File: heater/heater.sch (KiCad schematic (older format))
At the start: 9 parts, among them J1 power Input, J2 input uC, J3 thermostat, J4 to mcu, Q1 BC517

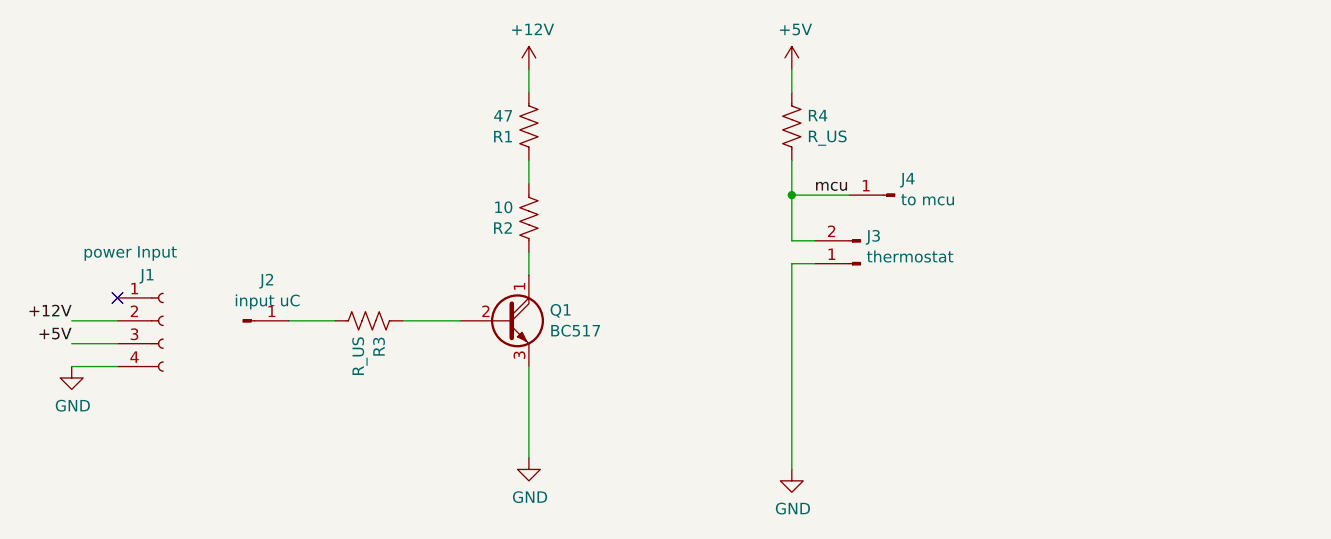
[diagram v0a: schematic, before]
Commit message: heater done
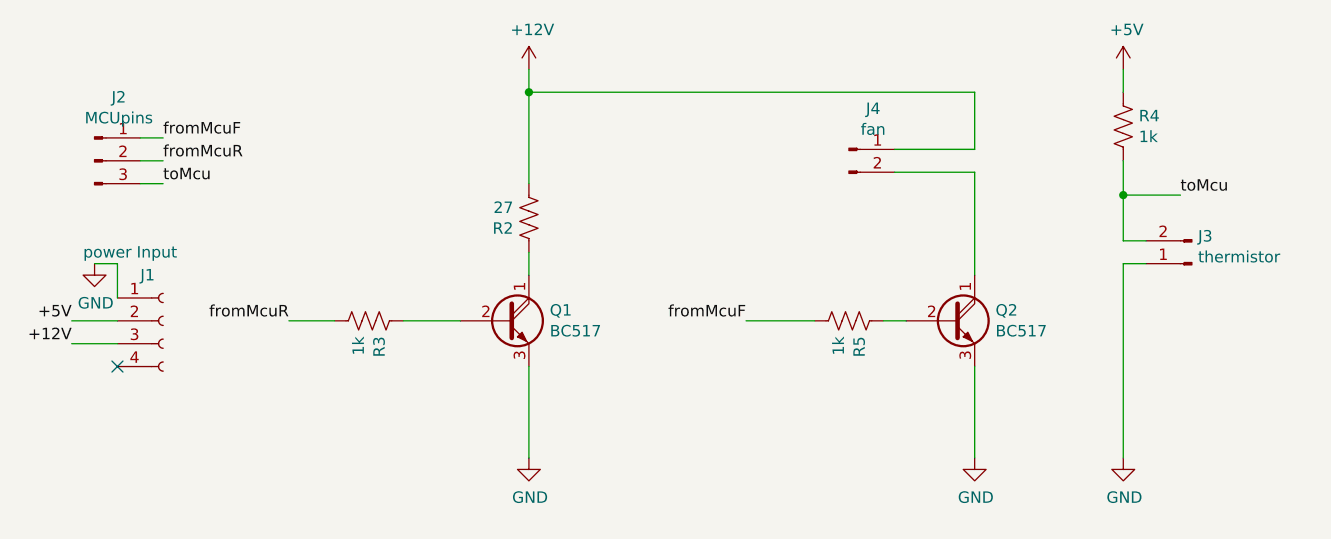
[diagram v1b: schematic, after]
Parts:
- removed J2: input uC, Socket_Strips:Socket_Strip_Straight_1x01_Pitch2.54mm, symbol Connector:Conn_01x01_Male
- removed J4: to mcu, Socket_Strips:Socket_Strip_Straight_1x01_Pitch2.54mm, symbol Connector:Conn_01x01_Male
- removed R1: 47, Resistors_THT:R_Axial_DIN0414_L11.9mm_D4.5mm_P15.24mm_Horizontal, symbol Device:R_US
- added J2: MCUpins, Connectors_JST:JST_XH_B03B-XH-A_03x2.50mm_Straight, symbol Connector:Conn_01x03_Male
- added J4: fan, Connectors_JST:JST_XH_B02B-XH-A_02x2.50mm_Straight, symbol Connector:Conn_01x02_Male
- added Q2: BC517, TO_SOT_Packages_THT:TO-92_Inline_Wide, symbol Transistor_BJT:BC517
- added R5: 1k, Resistors_SMD:R_0805_HandSoldering, symbol Device:R_US
- J1: footprint Connectors_JST:JST_EH_B04B-EH-A_04x2.50mm_Straight -> Connectors_JST:JST_XH_B04B-XH-A_04x2.50mm_Straight
- J3: value thermostat -> thermistor; footprint Socket_Strips:Socket_Strip_Straight_1x02_Pitch2.54mm -> Connectors_JST:JST_XH_B02B-XH-A_02x2.50mm_Straight
- R2: value 10 -> 27; footprint Resistors_THT:R_Axial_Power_L75.0mm_W9.0mm_P81.28mm -> Resistors_THT:R_Axial_Power_L38.0mm_W9.0mm_P40.64mm
- R3, R4: value R_US -> 1k
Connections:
- net +12V: now also J1.3 (Pin_3), R2.2, J4.1 (Pin_1); no longer J1.2 (Pin_2)
- net +5V: now also J1.2 (Pin_2); no longer J1.3 (Pin_3)
- net GND: now also J1.1 (Pin_1), Q2.3 (E); no longer J1.4 (Pin_4)
- net fromMcuR: now reaches R3.2
- net fromMcuR: now also J2.2 (Pin_2)
- net mcu renamed toMcu
- net toMcu: now also J2.3 (Pin_3)
- new net: J4.2 (Pin_2), Q2.1 (C)
- new net: Q2.2 (B), R5.1
- new net fromMcuF: J2.1 (Pin_1), R5.2
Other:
- moved on the sheet: J3, R4
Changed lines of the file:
@@
 P 3750 2050
 F 0 "R2" H 3818 2096 50  0000 L CNN
-F 1 "10" H 3818 2005 50  0000 L CNN
-F 2 "Resistors_THT:R_Axial_Power_L75.0mm_W9.0mm_P81.28mm" V 3790 2040 50  0001 C CNN
+F 1 "27" H 3818 2005 50  0000 L CNN
+F 2 "Resistors_THT:R_Axial_Power_L38.0mm_W9.0mm_P40.64mm" V 3790 2040 50  0001 C CNN
 F 3 "~" H 3750 2050 50  0001 C CNN
 	1    3750 2050
-	-1   0    0    1
-$EndComp
-$Comp
-L Device:R_US R1
-U 1 1 5C2F3120
-P 3750 1650
-F 0 "R1" H 3818 1696 50  0000 L CNN
-F 1 "47" H 3818 1605 50  0000 L CNN
-F 2 "Resistors_THT:R_Axial_DIN0414_L11.9mm_D4.5mm_P15.24mm_Horizontal" V 3790 1640 50  0001 C CNN
-F 3 "~" H 3750 1650 50  0001 C CNN
-	1    3750 1650
 	-1   0    0    1
 $EndComp
@@
 F 0 "J1" H 2050 2700 50  0000 L CNN
 F 1 "power Input" H 1800 2800 50  0000 L CNN
-F 2 "Connectors_JST:JST_EH_B04B-EH-A_04x2.50mm_Straight" H 2150 2500 50  0001 C CNN
+F 2 "Connectors_JST:JST_XH_B04B-XH-A_04x2.50mm_Straight" H 2150 2500 50  0001 C CNN
 F 3 "~" H 2150 2500 50  0001 C CNN
 	1    2150 2500
 	1    0    0    -1
 $EndComp
-Wire Wire Line
-	1950 2500 1750 2500
-Wire Wire Line
-	1950 2600 1750 2600
-Wire Wire Line
-	1950 2700 1750 2700
 Text Label 1750 2500 2    50   ~ 0
-+12V
-Text Label 1750 2600 2    50   ~ 0
 +5V
 $Comp
 L power:GND #PWR0101
 U 1 1 5C303485
-P 1750 2700
-F 0 "#PWR0101" H 1750 2450 50  0001 C CNN
-F 1 "GND" H 1755 2527 50  0000 C CNN
-F 2 "" H 1750 2700 50  0001 C CNN
-F 3 "" H 1750 2700 50  0001 C CNN
-	1    1750 2700
-	1    0    0    -1
-$EndComp
-NoConn ~ 1950 2400
+P 1850 2250
+F 0 "#PWR0101" H 1850 2000 50  0001 C CNN
+F 1 "GND" H 1855 2077 50  0000 C CNN
+F 2 "" H 1850 2250 50  0001 C CNN
+F 3 "" H 1850 2250 50  0001 C CNN
+	1    1850 2250
+	1    0    0    -1
+$EndComp
 $Comp
 L Transistor_BJT:BC517 Q1
@@
 $EndComp
 $Comp
-L Connector:Conn_01x01_Male J2
-U 1 1 5C307D7B
-P 2500 2500
-F 0 "J2" H 2606 2678 50  0000 C CNN
-F 1 "input uC" H 2606 2587 50  0000 C CNN
-F 2 "Socket_Strips:Socket_Strip_Straight_1x01_Pitch2.54mm" H 2500 2500 50  0001 C CNN
-F 3 "~" H 2500 2500 50  0001 C CNN
-	1    2500 2500
-	1    0    0    -1
-$EndComp
-$Comp
 L Device:R_US R3
 U 1 1 5C307DD4
 P 3050 2500
 F 0 "R3" H 3118 2546 50  0000 L CNN
-F 1 "R_US" H 3118 2455 50  0000 L CNN
+F 1 "1k" H 3118 2455 50  0000 L CNN
 F 2 "Resistors_SMD:R_0805_HandSoldering" V 3090 2490 50  0001 C CNN
 F 3 "~" H 3050 2500 50  0001 C CNN
@@
 	3200 2500 3450 2500
 Wire Wire Line
-	3750 1800 3750 1900
-Wire Wire Line
-	3750 2200 3750 2300
-Wire Wire Line
-	3750 1500 3750 1400
+	3750 2700 3750 3100
+$Comp
+L power:GND #PWR0103
+U 1 1 5C308243
+P 3750 3100
+F 0 "#PWR0103" H 3750 2850 50  0001 C CNN
+F 1 "GND" H 3755 2927 50  0000 C CNN
+F 2 "" H 3750 3100 50  0001 C CNN
+F 3 "" H 3750 3100 50  0001 C CNN
+	1    3750 3100
+	1    0    0    -1
+$EndComp
+$Comp
+L Connector:Conn_01x02_Male J3
+U 1 1 5C308B5A
+P 6650 2250
+F 0 "J3" H 6623 2130 50  0000 R CNN
+F 1 "thermistor" H 6623 2221 50  0000 R CNN
+F 2 "Connectors_JST:JST_XH_B02B-XH-A_02x2.50mm_Straight" H 6650 2250 50  0001 C CNN
+F 3 "~" H 6650 2250 50  0001 C CNN
+	1    6650 2250
+	-1   0    0    1
+$EndComp
+Wire Wire Line
+	6450 2250 6350 2250
+$Comp
+L Device:R_US R4
+U 1 1 5C336026
+P 6350 1650
+F 0 "R4" H 6418 1696 50  0000 L CNN
+F 1 "1k" H 6418 1605 50  0000 L CNN
+F 2 "Resistors_SMD:R_0805_HandSoldering" V 6390 1640 50  0001 C CNN
+F 3 "~" H 6350 1650 50  0001 C CNN
+	1    6350 1650
+	1    0    0    -1
+$EndComp
+$Comp
+L power:GND #PWR0104
+U 1 1 5C3360BC
+P 6350 3100
+F 0 "#PWR0104" H 6350 2850 50  0001 C CNN
+F 1 "GND" H 6355 2927 50  0000 C CNN
+F 2 "" H 6350 3100 50  0001 C CNN
+F 3 "" H 6350 3100 50  0001 C CNN
+	1    6350 3100
+	1    0    0    -1
+$EndComp
+Wire Wire Line
+	6450 2150 6350 2150
+Wire Wire Line
+	6350 2150 6350 1950
+$Comp
+L power:+5V #PWR0105
+U 1 1 5C33660C
+P 6350 1400
+F 0 "#PWR0105" H 6350 1250 50  0001 C CNN
+F 1 "+5V" H 6365 1573 50  0000 C CNN
+F 2 "" H 6350 1400 50  0001 C CNN
+F 3 "" H 6350 1400 50  0001 C CNN
+	1    6350 1400
+	1    0    0    -1
+$EndComp
+Wire Wire Line
+	6350 1400 6350 1500
+Wire Wire Line
+	6350 1950 6600 1950
+Connection ~ 6350 1950
+Text Label 6600 1950 0    50   ~ 0
+toMcu
+Text Label 2700 2500 2    50   ~ 0
+fromMcuR
+Wire Wire Line
+	2050 1800 2150 1800
+Wire Wire Line
+	2050 1900 2150 1900
+Text Label 2150 1800 0    50   ~ 0
+fromMcuR
+Text Label 2150 1900 0    50   ~ 0
+toMcu
+$Comp
+L Transistor_BJT:BC517 Q2
+U 1 1 5C346CA2
+P 5600 2500
+F 0 "Q2" H 5791 2546 50  0000 L CNN
+F 1 "BC517" H 5791 2455 50  0000 L CNN
+F 2 "TO_SOT_Packages_THT:TO-92_Inline_Wide" H 5800 2425 50  0001 L CIN
+F 3 "http://www.fairchildsemi.com/ds/BC/BC517.pdf" H 5600 2500 50  0001 L CNN
+	1    5600 2500
+	1    0    0    -1
+$EndComp
+$Comp
+L power:GND #PWR0106
+U 1 1 5C34725E
+P 5700 3100
+F 0 "#PWR0106" H 5700 2850 50  0001 C CNN
+F 1 "GND" H 5705 2927 50  0000 C CNN
+F 2 "" H 5700 3100 50  0001 C CNN
+F 3 "" H 5700 3100 50  0001 C CNN
+	1    5700 3100
+	1    0    0    -1
+$EndComp
+Wire Wire Line
+	5700 2700 5700 3100
+$Comp
+L Device:R_US R5
+U 1 1 5C3474DA
+P 5150 2500
+F 0 "R5" H 5218 2546 50  0000 L CNN
+F 1 "1k" H 5218 2455 50  0000 L CNN
+F 2 "Resistors_SMD:R_0805_HandSoldering" V 5190 2490 50  0001 C CNN
+F 3 "~" H 5150 2500 50  0001 C CNN
+	1    5150 2500
+	0    1    1    0
+$EndComp
+Wire Wire Line
+	5300 2500 5400 2500
+Wire Wire Line
+	6350 1950 6350 1800
+Wire Wire Line
+	5000 2500 4700 2500
+Text Label 4700 2500 2    50   ~ 0
+fromMcuF
+Wire Wire Line
+	6350 2250 6350 3100
+$Comp
+L Connector:Conn_01x02_Male J4
+U 1 1 5C34ABB8
+P 5150 1750
+F 0 "J4" H 5256 1928 50  0000 C CNN
+F 1 "fan" H 5256 1837 50  0000 C CNN
+F 2 "Connectors_JST:JST_XH_B02B-XH-A_02x2.50mm_Straight" H 5150 1750 50  0001 C CNN
+F 3 "~" H 5150 1750 50  0001 C CNN
+	1    5150 1750
+	1    0    0    -1
+$EndComp
+Wire Wire Line
+	5700 2300 5700 1850
+Wire Wire Line
+	5700 1850 5350 1850
+Text Label 1750 2600 2    50   ~ 0
++12V
 $Comp
 L power:+12V #PWR0102
@@
 $EndComp
 Wire Wire Line
-	3750 2700 3750 3100
-$Comp
-L power:GND #PWR0103
-U 1 1 5C308243
-P 3750 3100
-F 0 "#PWR0103" H 3750 2850 50  0001 C CNN
-F 1 "GND" H 3755 2927 50  0000 C CNN
-F 2 "" H 3750 3100 50  0001 C CNN
-F 3 "" H 3750 3100 50  0001 C CNN
-	1    3750 3100
-	1    0    0    -1
-$EndComp
-$Comp
-L Connector:Conn_01x02_Male J3
-U 1 1 5C308B5A
-P 5200 2250
-F 0 "J3" H 5173 2130 50  0000 R CNN
-F 1 "thermostat" H 5173 2221 50  0000 R CNN
-F 2 "Socket_Strips:Socket_Strip_Straight_1x02_Pitch2.54mm" H 5200 2250 50  0001 C CNN
-F 3 "~" H 5200 2250 50  0001 C CNN
-	1    5200 2250
-	-1   0    0    1
-$EndComp
-Wire Wire Line
-	5000 2250 4900 2250
-$Comp
-L Device:R_US R4
-U 1 1 5C336026
-P 4900 1650
-F 0 "R4" H 4968 1696 50  0000 L CNN
-F 1 "R_US" H 4968 1605 50  0000 L CNN
-F 2 "Resistors_SMD:R_0805_HandSoldering" V 4940 1640 50  0001 C CNN
-F 3 "~" H 4900 1650 50  0001 C CNN
-	1    4900 1650
-	1    0    0    -1
-$EndComp
-$Comp
-L power:GND #PWR0104
-U 1 1 5C3360BC
-P 4900 3150
-F 0 "#PWR0104" H 4900 2900 50  0001 C CNN
-F 1 "GND" H 4905 2977 50  0000 C CNN
-F 2 "" H 4900 3150 50  0001 C CNN
-F 3 "" H 4900 3150 50  0001 C CNN
-	1    4900 3150
-	1    0    0    -1
-$EndComp
-Wire Wire Line
-	5000 2150 4900 2150
-Wire Wire Line
-	4900 2150 4900 1950
-Wire Wire Line
-	4900 2250 4900 3150
-$Comp
-L power:+5V #PWR0105
-U 1 1 5C33660C
-P 4900 1400
-F 0 "#PWR0105" H 4900 1250 50  0001 C CNN
-F 1 "+5V" H 4915 1573 50  0000 C CNN
-F 2 "" H 4900 1400 50  0001 C CNN
-F 3 "" H 4900 1400 50  0001 C CNN
-	1    4900 1400
-	1    0    0    -1
-$EndComp
-Wire Wire Line
-	4900 1400 4900 1500
-Wire Wire Line
-	4900 1950 5150 1950
-Connection ~ 4900 1950
-Wire Wire Line
-	4900 1950 4900 1800
-Text Label 5000 1950 0    50   ~ 0
-mcu
-$Comp
-L Connector:Conn_01x01_Male J4
-U 1 1 5C336DF5
-P 5350 1950
-F 0 "J4" H 5323 1880 50  0000 R CNN
-F 1 "to mcu" H 5323 1971 50  0000 R CNN
-F 2 "Socket_Strips:Socket_Strip_Straight_1x01_Pitch2.54mm" H 5350 1950 50  0001 C CNN
-F 3 "~" H 5350 1950 50  0001 C CNN
-	1    5350 1950
-	-1   0    0    1
-$EndComp
+	5350 1750 5700 1750
+Wire Wire Line
+	5700 1750 5700 1500
+Wire Wire Line
+	5700 1500 3750 1500
+Wire Wire Line
+	3750 1400 3750 1500
+Wire Wire Line
+	3750 1500 3750 1900
+Connection ~ 3750 1500
+Wire Wire Line
+	3750 2200 3750 2300
+$Comp
+L Connector:Conn_01x03_Male J2
+U 1 1 5C350621
+P 1850 1800
+F 0 "J2" H 1956 2078 50  0000 C CNN
+F 1 "MCUpins" H 1956 1987 50  0000 C CNN
+F 2 "Connectors_JST:JST_XH_B03B-XH-A_03x2.50mm_Straight" H 1850 1800 50  0001 C CNN
+F 3 "~" H 1850 1800 50  0001 C CNN
+	1    1850 1800
+	1    0    0    -1
+$EndComp
+Wire Wire Line
+	2050 1700 2150 1700
+Text Label 2150 1700 0    50   ~ 0
+fromMcuF
+NoConn ~ 1950 2700
+Wire Wire Line
+	1750 2600 1950 2600
+Wire Wire Line
+	1750 2500 1950 2500
+Wire Wire Line
+	1950 2400 1950 2250
+Wire Wire Line
+	1950 2250 1850 2250
 $EndSCHEMATC
